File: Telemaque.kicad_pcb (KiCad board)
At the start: 2 copper layers, 100.4 x 50 mm, 75 parts, among them J1 Test, J2 Test, J3 Test, J4 Test, J5 Conn_01x01, J6 Conn_01x01, J7 Conn_01x01, P1 CONN_01X03, P2 CONN_01X10, P3 SMA, P4 CONN_01X05, P5 SMA, U1 LMC6482, U2 LD1117STR, U3 LD1117S50TR, U4 ACS723LLCTR-40AU-T, U5 LD1117S50TR, U6 LMC6482

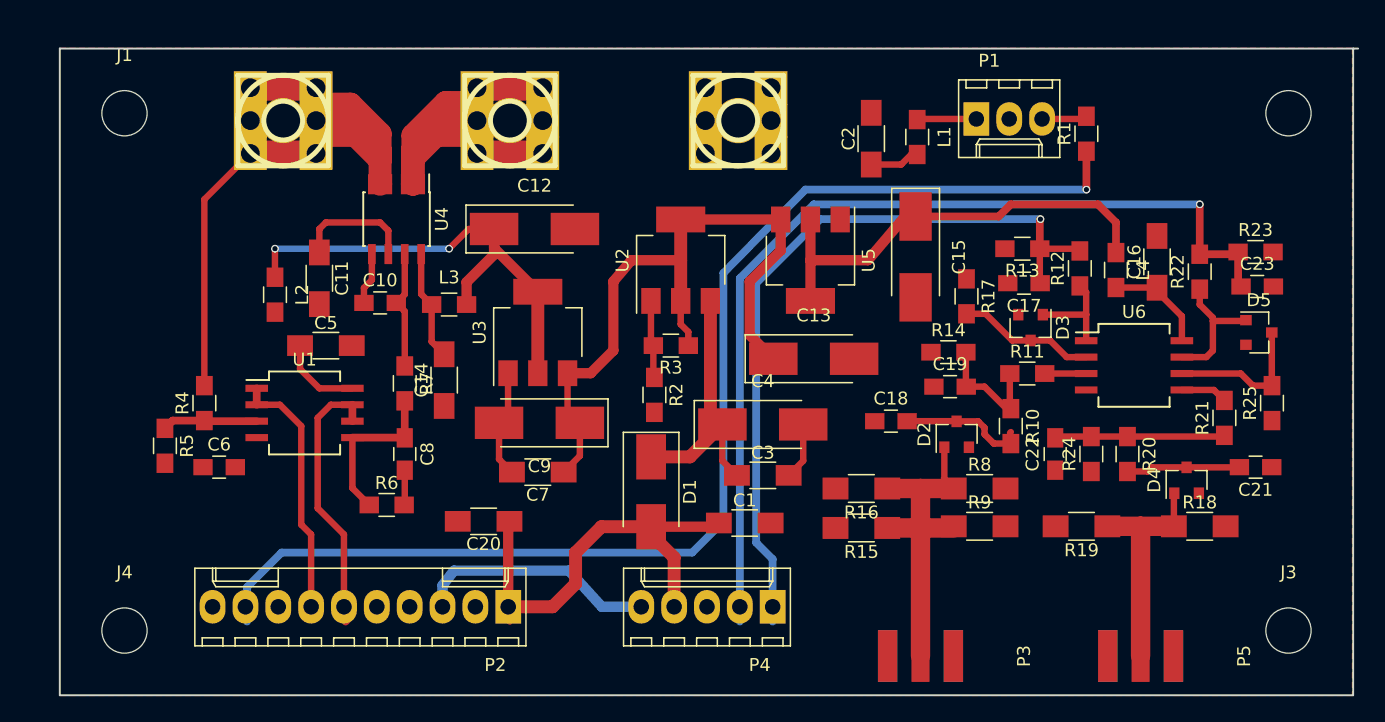
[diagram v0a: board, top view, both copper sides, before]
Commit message: Add files via upload
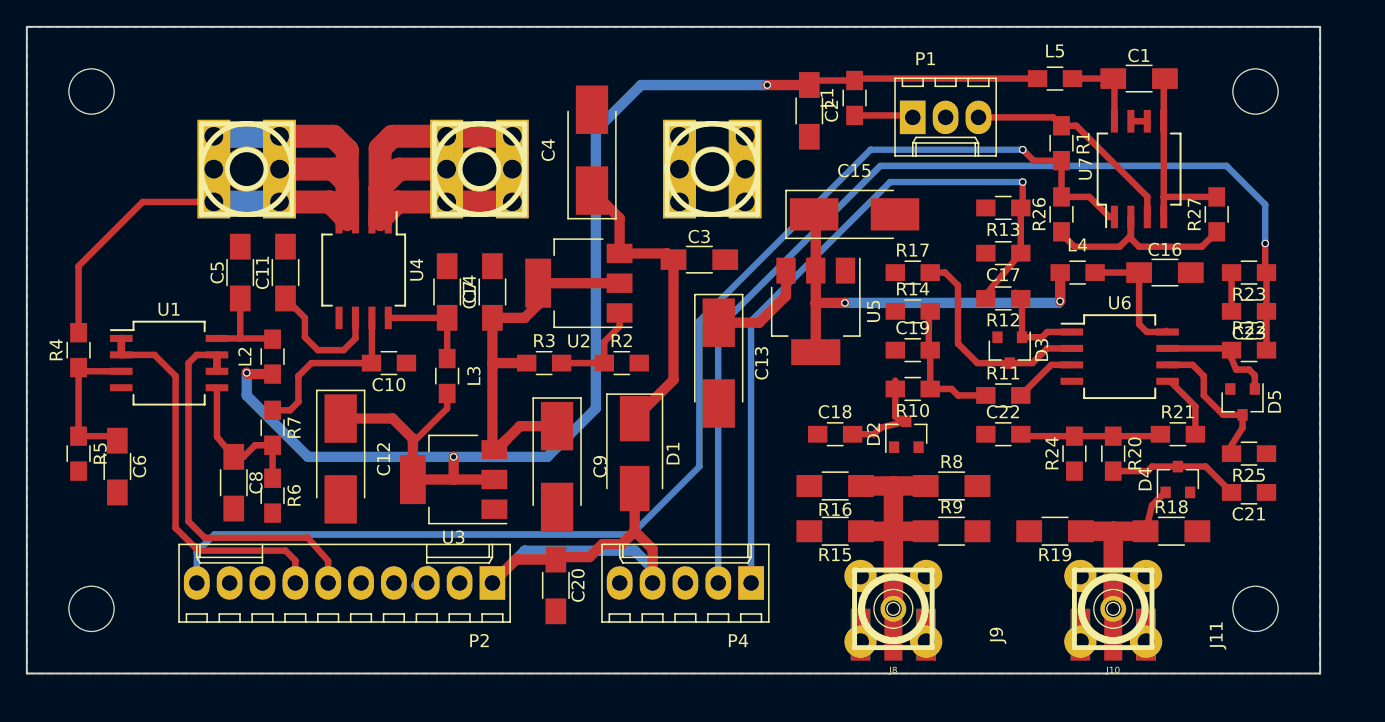
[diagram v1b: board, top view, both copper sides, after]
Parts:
- removed P3, P5: SMA, SMA_PINS:SMA_EDGE_NRW
- added J10: Conn_Coaxial, SMA_PINS:SMA_PINS, F.Cu at (164.0, 125.0)
- added J11: Conn_Coaxial, SMA_PINS:SMA_EDGE_NRW, F.Cu at (164.0, 127.0)
- added J8: Conn_Coaxial, SMA_PINS:SMA_PINS, F.Cu at (147.0, 125.0)
- added J9: Conn_Coaxial, SMA_PINS:SMA_EDGE_NRW, F.Cu at (147.0, 127.0)
- added L5: L_Core_Ferrite_Small, Inductors_SMD:L_0805_HandSoldering, F.Cu at (159.5, 84.0)
- added R26: R, Resistors_SMD:R_0805_HandSoldering, F.Cu at (160.0, 94.5)
- added R27: R, Resistors_SMD:R_0805_HandSoldering, F.Cu at (172.0, 94.5)
- added U7: LMC6082, Housings_SOIC:SO-8_5.3x6.2mm_Pitch1.27mm, F.Cu at (166.0, 91.0)
- C10, C17, C18, C19, C21, C22, C23: footprint Capacitors_SMD:C_0805_HandSoldering -> Resistors_SMD:R_0805_HandSoldering
- C6, C8: footprint Capacitors_SMD:C_0805_HandSoldering -> Capacitors_SMD:C_1206_HandSoldering
- J2: moved to F.Cu
- R1: value 2K -> R
- U4: footprint Housings_SOIC:SOIC-8_3.9x4.9mm_Pitch1.27mm -> Housings_SOIC:SO-8_5.3x6.2mm_Pitch1.27mm
- moved J2 92.6 mm to (85.0, 85.0)
- moved J3 92.6 mm to (85.0, 125.0)
- moved J1 87.5 mm to (175.0, 85.0)
- moved J4 87.5 mm to (175.0, 125.0)
- moved C1 45.9 mm to (166.0, 84.0)
- moved C4 25.0 mm to (123.7, 89.5), turned to 90 degrees
- moved C12 23.3 mm to (104.3, 113.4), turned to 270 degrees
- moved C3 17.4 mm to (132.0, 98.0)
- moved C7 14.4 mm to (116.0, 100.5), turned to 90 degrees
- moved C8 13.4 mm to (96.0, 115.2)
- moved U3 13.1 mm to (113.0, 115.0), turned to 180 degrees
- moved U1 11.2 mm to (91.0, 106.0)
- moved R7 10.8 mm to (99.0, 111.0)
- moved R4 10.6 mm to (84.0, 105.0)
- moved R3 9.89 mm to (120.0, 106.0), turned to 0 degrees
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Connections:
- C1 pad 1: +12V -> Net-(C1-Pad1)
- P2 pad 10: GND -> Net-(P2-Pad10)
- P2 pad 9: Net-(P2-Pad9) -> GND
- R1 pad 1: Net-(P2-Pad9) -> Net-(P1-Pad3)
- R1 pad 2: Net-(P1-Pad3) -> Net-(P2-Pad10)
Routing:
- net Net-(P2-Pad10): track 0.00 -> 97.8 mm, vias 0 -> 1
- net Net-(P2-Pad9): track 94.5 -> 0.00 mm, vias 1 -> 0
- net +5VA: track 43.0 -> 114.7 mm, vias 2 -> 3
- net Net-(C13-Pad1): track 55.7 -> 38.8 mm
- net Net-(R26-Pad1): track 0.00 -> 16.8 mm
- net Net-(P2-Pad3): track 18.8 -> 2.25 mm
- net Net-(P1-Pad3): track 3.51 -> 17.7 mm
- net Net-(J5-Pad1): track 73.6 -> 59.4 mm
- net Net-(P2-Pad7): track 19.7 -> 29.9 mm
- net Net-(P2-Pad6): track 20.0 -> 29.8 mm
- net Net-(J6-Pad1): track 50.7 -> 41.4 mm
- net Net-(D2-Pad2): track 26.7 -> 19.5 mm
- net Net-(C1-Pad1): track 0.00 -> 6.62 mm
- net Net-(D3-Pad1): track 10.7 -> 17.2 mm
- net Net-(C23-Pad1): track 74.1 -> 80.1 mm
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- added copper zone on B.Cu, net GND
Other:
- board size 100.4 x 50 mm -> 100 x 50 mm
